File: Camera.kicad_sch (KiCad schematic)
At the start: 84 parts, among them J6 VJ1, Q3 BC857, Q4 2N7002, U11 LFE5U-85F-6BG381C, U12 TLV62569DBV, U13 TLV62569DBV, U14 TLV62569DBV, U8 MCP7940NT, Y3 32768Hz

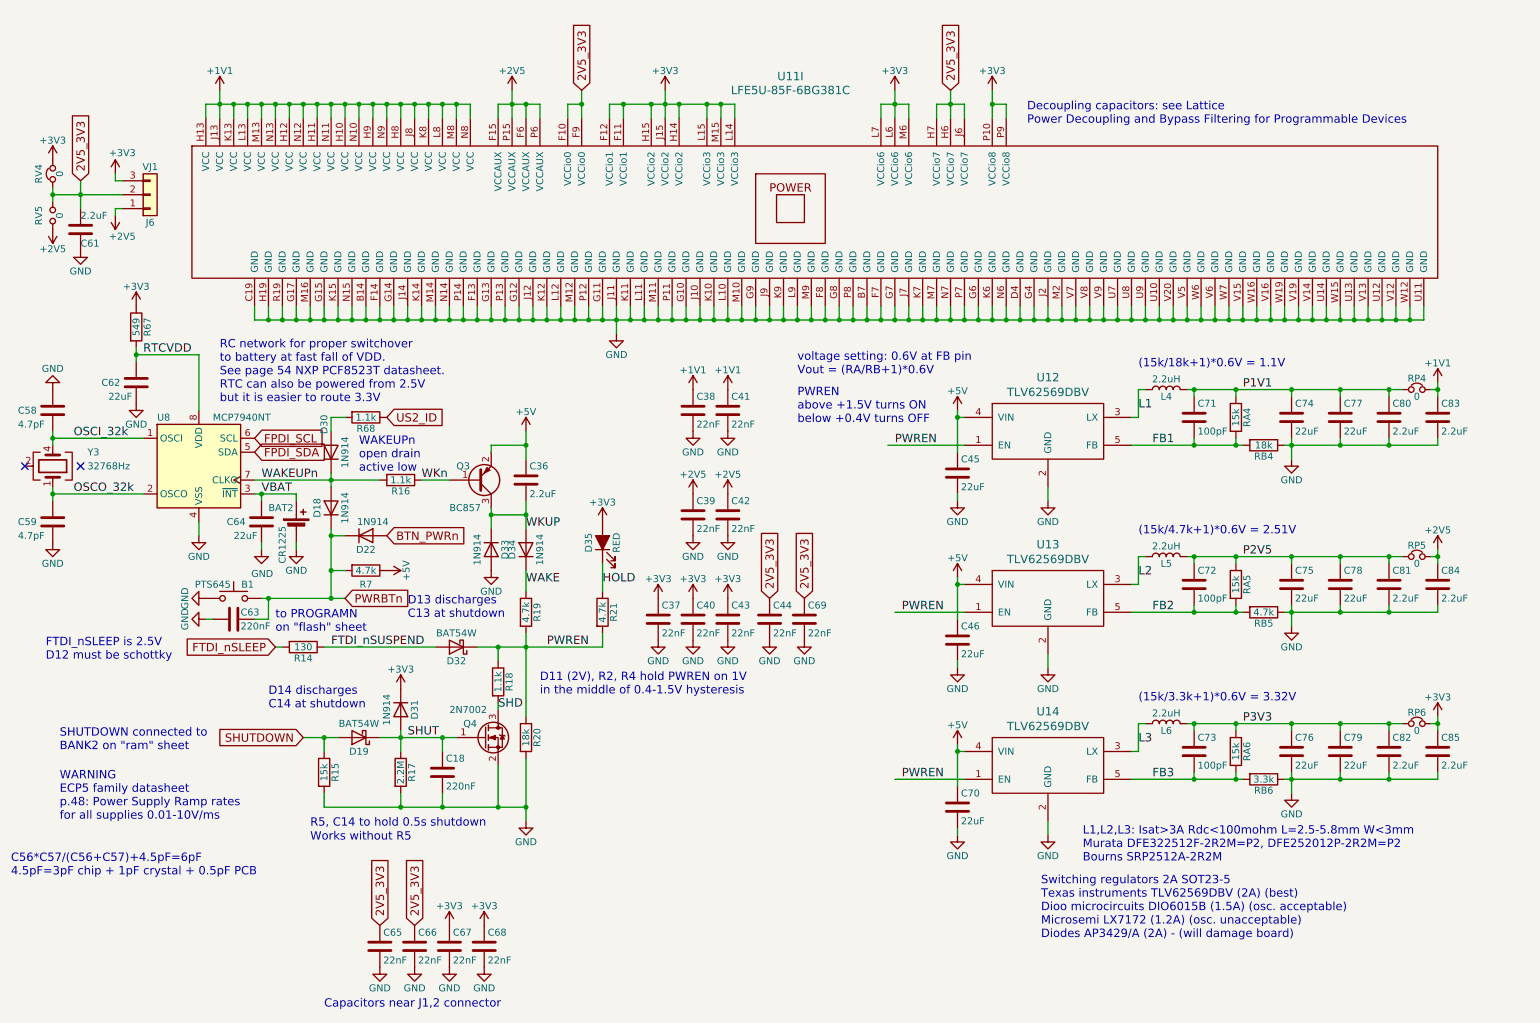
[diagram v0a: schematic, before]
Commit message: AI 1st attempt at add camera.
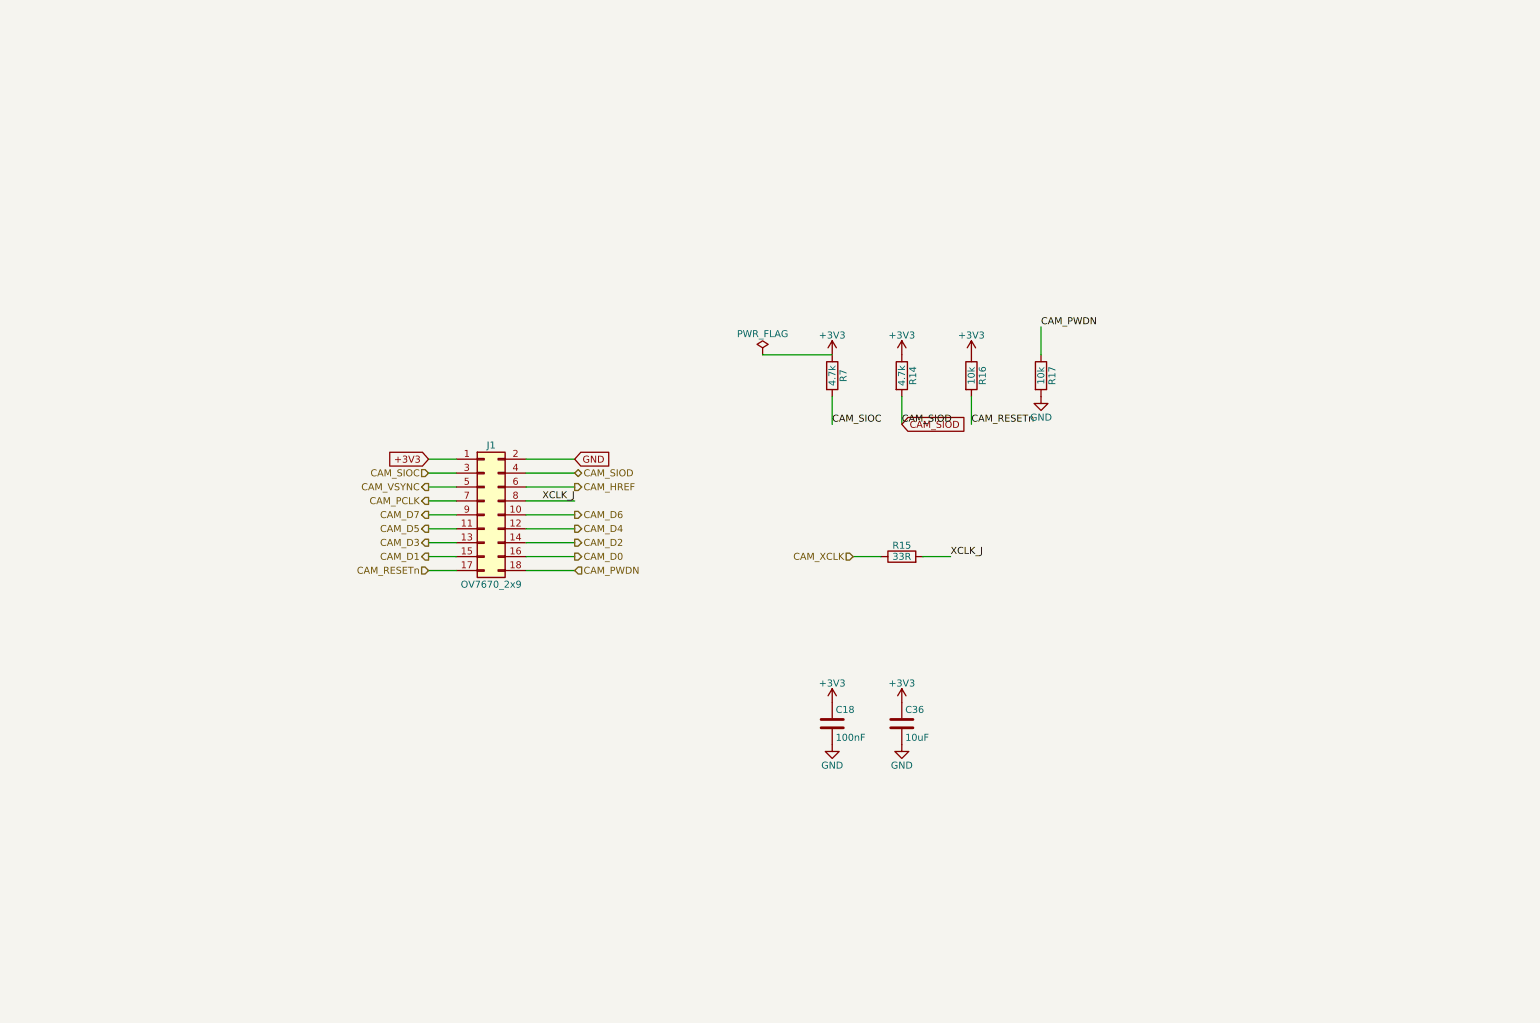
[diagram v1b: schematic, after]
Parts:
- removed B1: PTS645, Button_Switch_SMD:SW_SPST_PTS645, symbol Switch:SW_Push
- removed BAT2: CR1225, Keystone_3000_1x12mm-CoinCell:Keystone_3000_1x12mm-CoinCell, symbol Device:Battery_Cell
- removed C37, C38, C39, C40, C41, C42, C43, C44, C65, C66, C67, C68, C69: 22nF, Capacitor_SMD:C_0603_1608Metric, symbol Device:C
- removed C45, C46, C62, C64, C70, C74, C75, C76, C77, C78, C79: 22uF, Capacitor_SMD:C_0805_2012Metric, symbol Device:C
- removed C58, C59: 4.7pF, Capacitor_SMD:C_0603_1608Metric, symbol Device:C
- removed C61, C80, C81, C82, C83, C84, C85: 2.2uF, Capacitor_SMD:C_0805_2012Metric, symbol Device:C
- removed C63: 220nF, Capacitor_SMD:C_0603_1608Metric, symbol Device:C
- removed C71, C72, C73: 100pF, Capacitor_SMD:C_0603_1608Metric, symbol Device:C
- removed D18, D22, D30, D31, D33, D34: 1N914, Diode_SMD:D_SOD-323_HandSoldering, symbol Device:D
- removed D19, D32: BAT54W, Diode_SMD:D_SOD-323_HandSoldering, symbol Device:D_Schottky
- removed D35: RED, LED_SMD:LED_0805_2012Metric, symbol Device:LED_ALT
- removed J6: VJ1, Connector_PinHeader_2.54mm:PinHeader_1x03_P2.54mm_Vertical, symbol Connector_Generic:Conn_01x03
- removed L4, L5, L6: 2.2uH, L_1008_1210:L_1008_1210, symbol Device:L
- removed Q3: BC857, Package_TO_SOT_SMD:SOT-23, symbol Device:Q_PNP_BEC
- removed Q4: 2N7002, Package_TO_SOT_SMD:SOT-23, symbol Device:Q_NMOS_GSD
- removed R18, R68: 1.1k, Resistor_SMD:R_0603_1608Metric, symbol Device:R
- removed R19, R21, RB5: 4.7k, Resistor_SMD:R_0603_1608Metric, symbol Device:R
- removed R20, RB4: 18k, Resistor_SMD:R_0603_1608Metric, symbol Device:R
- removed R67: 549, Resistor_SMD:R_0603_1608Metric, symbol Device:R
- removed RA4, RA5, RA6: 15k, Resistor_SMD:R_0603_1608Metric, symbol Device:R
- removed RB6: 3.3k, Resistor_SMD:R_0603_1608Metric, symbol Device:R
- removed RP4, RP5, RP6: 0, jumper:R_0805_2012Metric_Pad1.29x1.40mm_HandSolder_Jumper_NC, symbol Device:Jumper_NC_Small
- removed RV4: 0, Resistor_SMD:R_0805_2012Metric_Pad1.29x1.40mm_HandSolder, symbol Device:Jumper_NC_Small
- removed RV5: 0, Resistor_SMD:R_0805_2012Metric_Pad1.29x1.40mm_HandSolder, symbol Device:Jumper_NO_Small
- removed U11: LFE5U-85F-6BG381C, lfe5bg381:BGA-381_pitch0.8mm_dia0.4mm, symbol lfe5bg381:LFE5UM-85F-6BG381C
- removed U12, U13, U14: TLV62569DBV, TSOT-25:TSOT-25, symbol dcdc:DCDC
- removed U8: MCP7940NT, SOT96-1:SOT96-1, symbol Timer_RTC:PCF8563T
- removed Y3: 32768Hz, abs07:Crystal_SMD_ABS07, symbol Device:Crystal_GND23
- added J1: OV7670_2x9, Connector_PinSocket_2.54mm:PinSocket_2x09_P2.54mm_Vertical, symbol Connector_Generic:Conn_02x09_Odd_Even
- C18: value 220nF -> 100nF; footprint Capacitor_SMD:C_0603_1608Metric -> Capacitor_SMD:C_0402_1005Metric; Digikey 1276-1112-1-ND -> (none); Koncar FC002 -> (none); LCSC C326805 -> C1525; MNF1_URL www.yageo.com -> (none); MPN CC0603KRX7R8BB224 -> (none); Mouse_r1 81-GCM188R71E224K55D -> (none); Mouser 603-CC603KRX7R6BB224 -> (none); Newark 82AC9347 -> (none); Side TB -> (none)
- C36: value 2.2uF -> 10uF; Digike_y2 1276-2903-1-ND -> (none); Digikey 587-5918-1-ND -> (none); Koncar FC001 -> (none); LCSC C87995 -> C15850; MPN CC0805MRX5R6BB225 -> (none); Mouse_r1 80-C0805C225K4R3123 -> (none); Mouse_r2 603-CC805MRX5R6BB225 -> (none); Mouser 187-CL21B225KOFNNNG -> (none); Newar_k2 70K9141 -> (none); Newark 73AH0064 -> (none)
- R14: value 130 -> 4.7k; footprint Resistor_SMD:R_0603_1608Metric -> Resistor_SMD:R_0402_1005Metric; LCSC (none) -> C25900
- R15: value 15k -> 33R; footprint Resistor_SMD:R_0603_1608Metric -> Resistor_SMD:R_0402_1005Metric; LCSC (none) -> C25105
- R16: value 1.1k -> 10k; footprint Resistor_SMD:R_0603_1608Metric -> Resistor_SMD:R_0402_1005Metric; LCSC (none) -> C25744
- R17: value 2.2M -> 10k; footprint Resistor_SMD:R_0603_1608Metric -> Resistor_SMD:R_0402_1005Metric; Digikey P2.20MHCT-ND -> (none); Koncar FR007 -> (none); LCSC C18679 -> C25744; MNF1_URL www.yageo.com -> (none); MPN RC0603FR-132M2L -> (none); Mouser 603-AC0603FR-072M2L -> (none); Newark 89M6741 -> (none)
- R7: footprint Resistor_SMD:R_0603_1608Metric -> Resistor_SMD:R_0402_1005Metric; LCSC (none) -> C25900; MPN AC0603FR-104K7L -> (none)
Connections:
- net +5V is gone; now on net +3V3: C36.1, R7.1
- net FTDI_nSUSPEND is gone; now on net +3V3: R14.1
- net WKUP is gone; now on net GND: C36.2
- net WKn is gone; now on net +3V3: R16.1
- net +3V3: now also C18.1, J1.1 (Pin_1)
- net GND: now also J1.2 (Pin_2); no longer R15.2
- net FTDI_nSLEEP renamed CAM_SIOD
- net CAM_SIOD: now also J1.4 (Pin_4)
- net PWRBTn renamed CAM_SIOC
- net CAM_SIOC: now also J1.3 (Pin_3)
- net SHUT renamed CAM_PWDN
- net CAM_PWDN: now also J1.18 (Pin_18); no longer C18.1
- net SHUTDOWN renamed CAM_XCLK
- net WAKEUPn renamed CAM_RESETn
- net CAM_RESETn: now also J1.17 (Pin_17)
- new net CAM_D0: J1.16 (Pin_16)
- new net CAM_D1: J1.15 (Pin_15)
- new net CAM_D2: J1.14 (Pin_14)
- new net CAM_D3: J1.13 (Pin_13)
- new net CAM_D4: J1.12 (Pin_12)
- new net CAM_D5: J1.11 (Pin_11)
- new net CAM_D6: J1.10 (Pin_10)
- new net CAM_D7: J1.9 (Pin_9)
- new net CAM_HREF: J1.6 (Pin_6)
- new net CAM_PCLK: J1.7 (Pin_7)
- new net CAM_VSYNC: J1.5 (Pin_5)
- new net XCLK_J: J1.8 (Pin_8), R15.2
- no-connect marks 2 -> 0
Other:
- note removed: "(15k/18k+1)*0.6V = 1.1V"
- note removed: "(15k/3.3k+1)*0.6V = 3.32V"
- note removed: "(15k/4.7k+1)*0.6V = 2.51V"
- note removed: "C56*C57/(C56+C57)+4.5pF=6pF 4.5pF=3pF chip + 1pF crystal + 0.5pF PCB"
- note removed: "Capacitors near J1,2 connector"
- note removed: "D11 (2V), R2, R4 hold PWREN on 1V in the middle of 0.4-1.5V hysteresis"
- note removed: "D13 discharges C13 at shutdown"
- note removed: "D14 discharges C14 at shutdown"
- note removed: "Decoupling capacitors: see Lattice Power Decoupling and Bypass Filtering for Programmable Devices"
- note removed: "FTDI_nSLEEP is 2.5V D12 must be schottky"
- note removed: "L1,L2,L3: Isat>3A Rdc<100mohm L=2.5-5.8mm W<3mm Murata DFE322512F-2R2M=P2, DFE252012P-2R2M=P2 Bourns SRP2512A-2R2M"
- note removed: "PWREN above +1.5V turns ON below +0.4V turns OFF"
- note removed: "R5, C14 to hold 0.5s shutdown"
- note removed: "RC network for proper switchover to battery at fast fall of VDD. See page 54 NXP PCF8523T datasheet. RTC can also be powered from 2.5V but it is easier to route 3.3V"
- note removed: "SHUTDOWN connected to BANK2 on "ram" sheet"
- note removed: "Switching regulators 2A SOT23-5 Texas instruments TLV62569DBV (2A) (best) Dioo microcircuits DIO6015B (1.5A) (osc. acceptable) Microsemi LX7172 (1.2A) (osc. unacceptable) Diodes AP3429/A (2A) - (will damage board)"
- note removed: "WAKEUPn open drain active low"
- note removed: "WARNING ECP5 family datasheet p.48: Power Supply Ramp rates for all supplies 0.01-10V/ms"
- note removed: "Works without R5"
- note removed: "to PROGRAMN on "flash" sheet"
- note removed: "voltage setting: 0.6V at FB pin Vout = (RA/RB+1)*0.6V"
